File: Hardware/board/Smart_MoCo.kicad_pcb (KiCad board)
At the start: 4 copper layers, 26.9 x 39.9 mm, 37 parts, among them J1 Conn_01x02, J2 Conn_01x04, J3 Conn_01x02, J4 Conn_01x02, J5 Conn_01x04, J6 1722861102, J7 1722861102, U1 STM32F042F6Px, U2 VNH5019A-E, U3 SN65HVD232, U4 AP62200WU

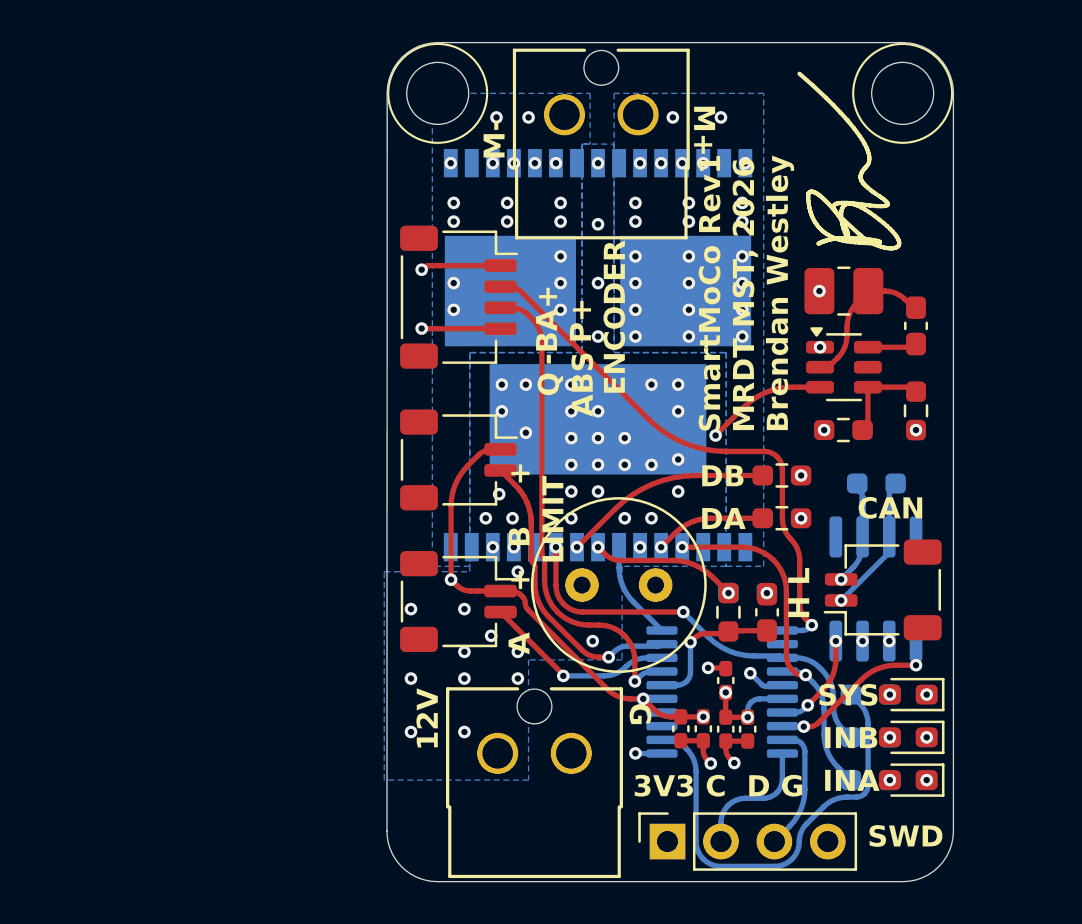
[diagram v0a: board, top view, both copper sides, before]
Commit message: Redesign hardware
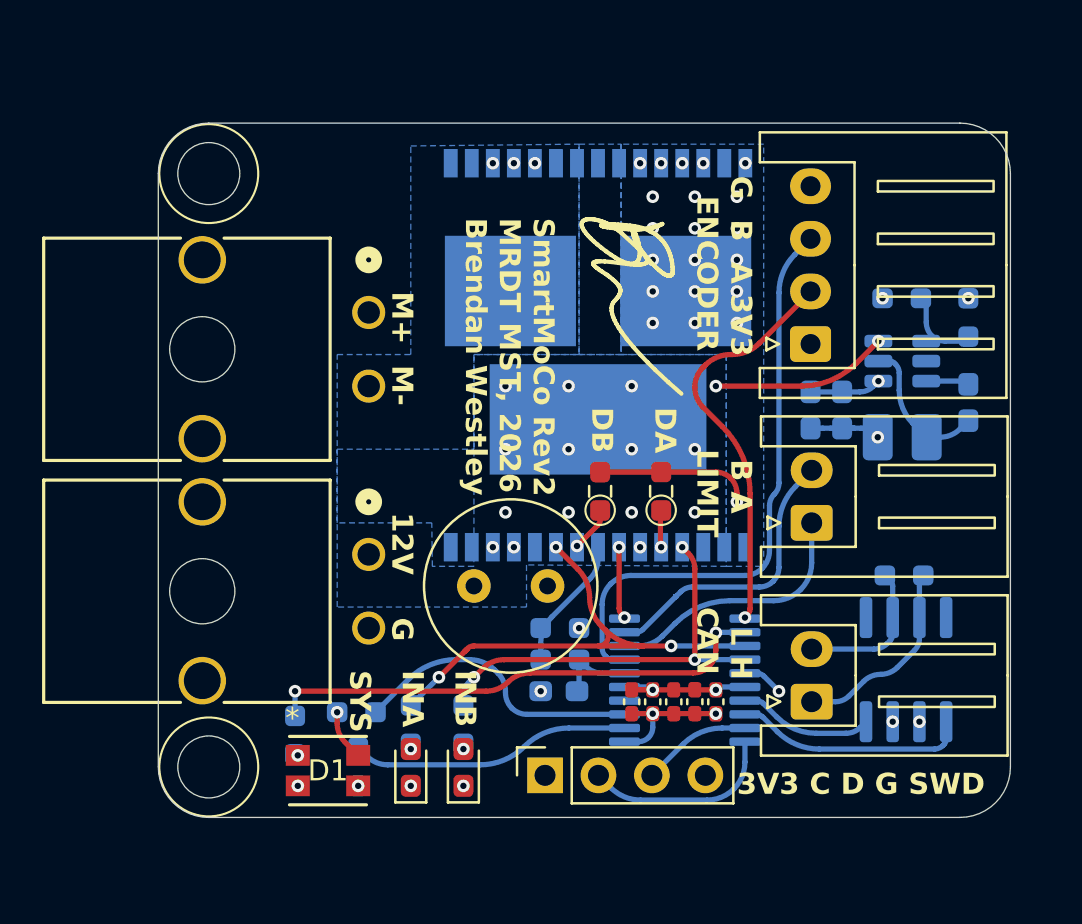
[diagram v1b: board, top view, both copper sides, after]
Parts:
- removed the J4 at (145.8, 78.5)
- removed J7: 1722861102, MRDT_Connectors:CONN_SD-172286-1000_02_MOL
- added C4: 22uF, Capacitor_SMD:C_0603_1608Metric_Pad1.08x0.95mm_HandSolder, B.Cu at (164.0, 76.1)
- added C5: 22uF, Capacitor_SMD:C_0603_1608Metric_Pad1.08x0.95mm_HandSolder, B.Cu at (162.5, 76.1)
- added J5: 1723103102, MRDT_Connectors:CONN_1723102000_02_MOL, F.Cu at (141.5, 83.0)
- added R10: 1k, Resistor_SMD:R_0603_1608Metric_Pad0.98x0.95mm_HandSolder, B.Cu at (141.0, 93.1)
- added R9: 1k, Resistor_SMD:R_0603_1608Metric_Pad0.98x0.95mm_HandSolder, B.Cu at (140.9, 90.5)
- C1, C3, L1, R1, R6, R7, U4: moved to B.Cu
- D1: value Red -> LED_RGBK; footprint LED_SMD:LED_0603_1608Metric_Pad1.05x0.95mm_HandSolder -> Smart_MoCo:PLCC4_3p5x2p8_SLD-L
- J1, J3: footprint Connector_JST:JST_SH_SM02B-SRSS-TB_1x02-1MP_P1.00mm_Horizontal -> Connector_JST:JST_XH_S2B-XH-A_1x02_P2.50mm_Horizontal
- J2: footprint Connector_JST:JST_SH_SM04B-SRSS-TB_1x04-1MP_P1.00mm_Horizontal -> Connector_JST:JST_XH_S4B-XH-A_1x04_P2.50mm_Horizontal
- J6: value 1722861102 -> 1723103102; footprint MRDT_Connectors:CONN_SD-172286-1000_02_MOL -> MRDT_Connectors:CONN_1723102000_02_MOL
- moved H1 46.0 mm to (133.9, 93.1)
- moved G*** 29.1 mm to (167.5, 67.0)
- moved D1 27.8 mm to (139.6, 93.3), turned to 0 degrees
- moved R8 27.4 mm to (138.0, 91.6), turned to -90 degrees
- moved D2 23.7 mm to (143.5, 93.1), turned to 90 degrees
- moved R12 21.8 mm to (143.5, 91.1), turned to -90 degrees
- moved D3 21.2 mm to (146.0, 93.1), turned to 90 degrees
- moved R11 19.5 mm to (146.0, 91.1), turned to -90 degrees
- moved J3 17.2 mm to (162.6, 81.5), turned to 90 degrees
- moved J2 16.9 mm to (162.5, 73.0), turned to 90 degrees
- moved J6 15.9 mm to (141.5, 71.5), turned to -90 degrees
- moved REF** 12.2 mm to (154.0, 71.0), turned to -90 degrees
- moved H2 11.5 mm to (133.9, 64.9)
- moved C1 10.6 mm to (150.5, 89.5), turned to 0 degrees
- moved R4 9.08 mm to (150.6, 86.5)
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- renumbered C8 to C10, C5 to C7, C4 to C8, C7 to C9, J5 to J4, R10 to R11, R9 to R12
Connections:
- D1 pad 1: GND -> Net-(D1-RA)
- D1 pad 2: Net-(D1-A) -> Net-(D1-GA)
- J3 pad 1: +3V3 -> LIM_A
- J3 pad 2: LIM_A -> LIM_B
- R8 pad 1: LED_STATUS -> LED_R
- R8 pad 2: Net-(D1-A) -> Net-(D1-RA)
- U1 pad 12: unconnected-(U1-PA6-Pad12) -> LED_R
- U1 pad 2: LED_STATUS -> LED_B
- U1 pad 3: unconnected-(U1-PF1-Pad3) -> LED_G
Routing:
- net LED_R: track 0.00 -> 24.2 mm, vias 0 -> 2
- net LED_STATUS: track 21.2 -> 0.00 mm
- net +3V3: track 31.3 -> 16.1 mm, vias 11 -> 6
- net LED_G: track 0.00 -> 14.1 mm
- net LED_B: track 0.00 -> 13.4 mm
- net Net-(U2-EN/DIAGB): track 9.98 -> 1.83 mm
- net ENC_A/PWM: track 26.1 -> 19.3 mm
- net IN_B: track 19.7 -> 24.9 mm, vias 2 -> 3
- net ENC_B: track 23.1 -> 27.8 mm, vias 1 -> 0
- net CS: track 6.95 -> 3.28 mm, vias 1 -> 0
- net Net-(U2-EN/DIAGA): track 5.28 -> 1.76 mm
- net LIM_A: track 9.17 -> 12.4 mm, vias 1 -> 0
- net SWCLK: track 6.51 -> 9.34 mm
- net IN_A: track 17.5 -> 20.2 mm, vias 2 -> 3
- net +12V: track 5.76 -> 8.43 mm, vias 46 -> 15
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- removed copper zone on In2.Cu, net /OUTB
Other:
- board size 26.9 x 39.9 mm -> 40.5 x 33 mm
- board text added: "3V3 C D G SWD"
- board text added: "B A LIMIT"
- board text added: "G B A 3V3 ENCODER"
- board text added: "L H CAN"
- board text added: "SmartMoCo Rev2 MRDT MST, 2026 Brendan Westley"
- board text removed: "-BA+ - P+ ENCODER"
- board text removed: "3V3 C D G"
- board text removed: "A + B + LIMIT"
- board text removed: "CAN"
- board text removed: "H L"
- board text removed: "Q ABS"
- board text removed: "SWD"
- board text removed: "SmartMoCo Rev1 MRDT MST, 2026 Brendan Westley"
